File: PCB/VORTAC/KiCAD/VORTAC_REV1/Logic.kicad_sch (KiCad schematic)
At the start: 28 parts, among them U1 TLV73333PDBV, U3 EE-SX3350, U4 TPS54335ADRCR, U7 EE-SX3350

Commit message: Fixed Library stuff
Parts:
- L2: footprint ToolChanger:L_Sunlord_MWSA0518_5.4x5.2mm -> Vortac:L_Sunlord_MWSA0518_5.4x5.2mm; LCSC C408412 -> C436530; LCSC ALT C436530 -> (none)
- U3, U7: footprint ToolChanger:SENSOR_EE-SX3350_OMR -> Vortac:SENSOR_EE-SX3350_OMR
- U4: footprint ToolChanger:VSON-10-1EP_3x3mm_P0.5mm_EP1.65x2.4mm_ThermalVias -> Vortac:VSON-10-1EP_3x3mm_P0.5mm_EP1.65x2.4mm_ThermalVias
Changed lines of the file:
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@@
 			)
 		)
-		(property "Footprint" "ToolChanger:L_Sunlord_MWSA0518_5.4x5.2mm"
+		(property "Footprint" "Vortac:L_Sunlord_MWSA0518_5.4x5.2mm"
 			(at 82.55 116.84 0)
 			(effects
@@
 			)
 		)
-		(property "LCSC" "C408412"
-			(at 82.55 116.84 90)
-			(effects
-				(font
-					(size 1.27 1.27)
-				)
-				(hide yes)
-			)
-		)
-		(property "LCSC ALT" "C436530"
+		(property "LCSC" "C436530"
 			(at 82.55 116.84 90)
 			(effects
@@
 			)
 		)
-		(property "Footprint" "ToolChanger:VSON-10-1EP_3x3mm_P0.5mm_EP1.65x2.4mm_ThermalVias"
+		(property "Footprint" "Vortac:VSON-10-1EP_3x3mm_P0.5mm_EP1.65x2.4mm_ThermalVias"
 			(at 66.04 133.35 0)
 			(effects
@@
 			)
 		)
-		(property "Footprint" "ToolChanger:SENSOR_EE-SX3350_OMR"
+		(property "Footprint" "Vortac:SENSOR_EE-SX3350_OMR"
 			(at 214.884 67.564 0)
 			(effects
@@
 			)
 		)
-		(property "Footprint" "ToolChanger:SENSOR_EE-SX3350_OMR"
+		(property "Footprint" "Vortac:SENSOR_EE-SX3350_OMR"
 			(at 214.884 44.704 0)
 			(effects

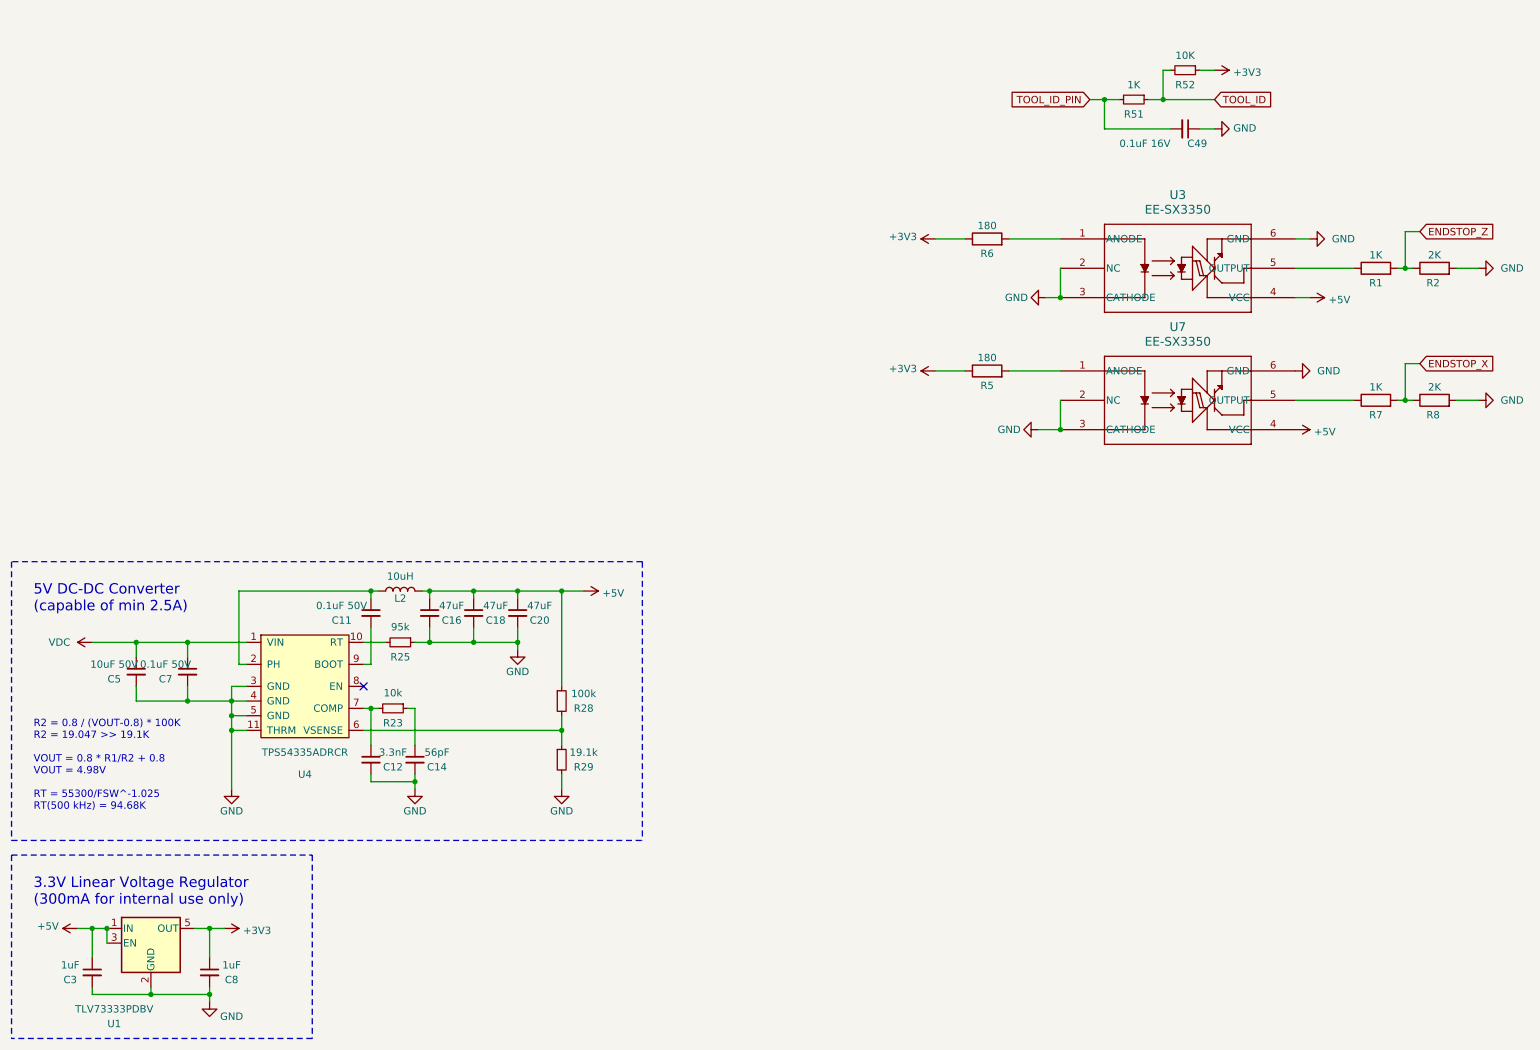
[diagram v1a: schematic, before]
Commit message: pls merge Jenno
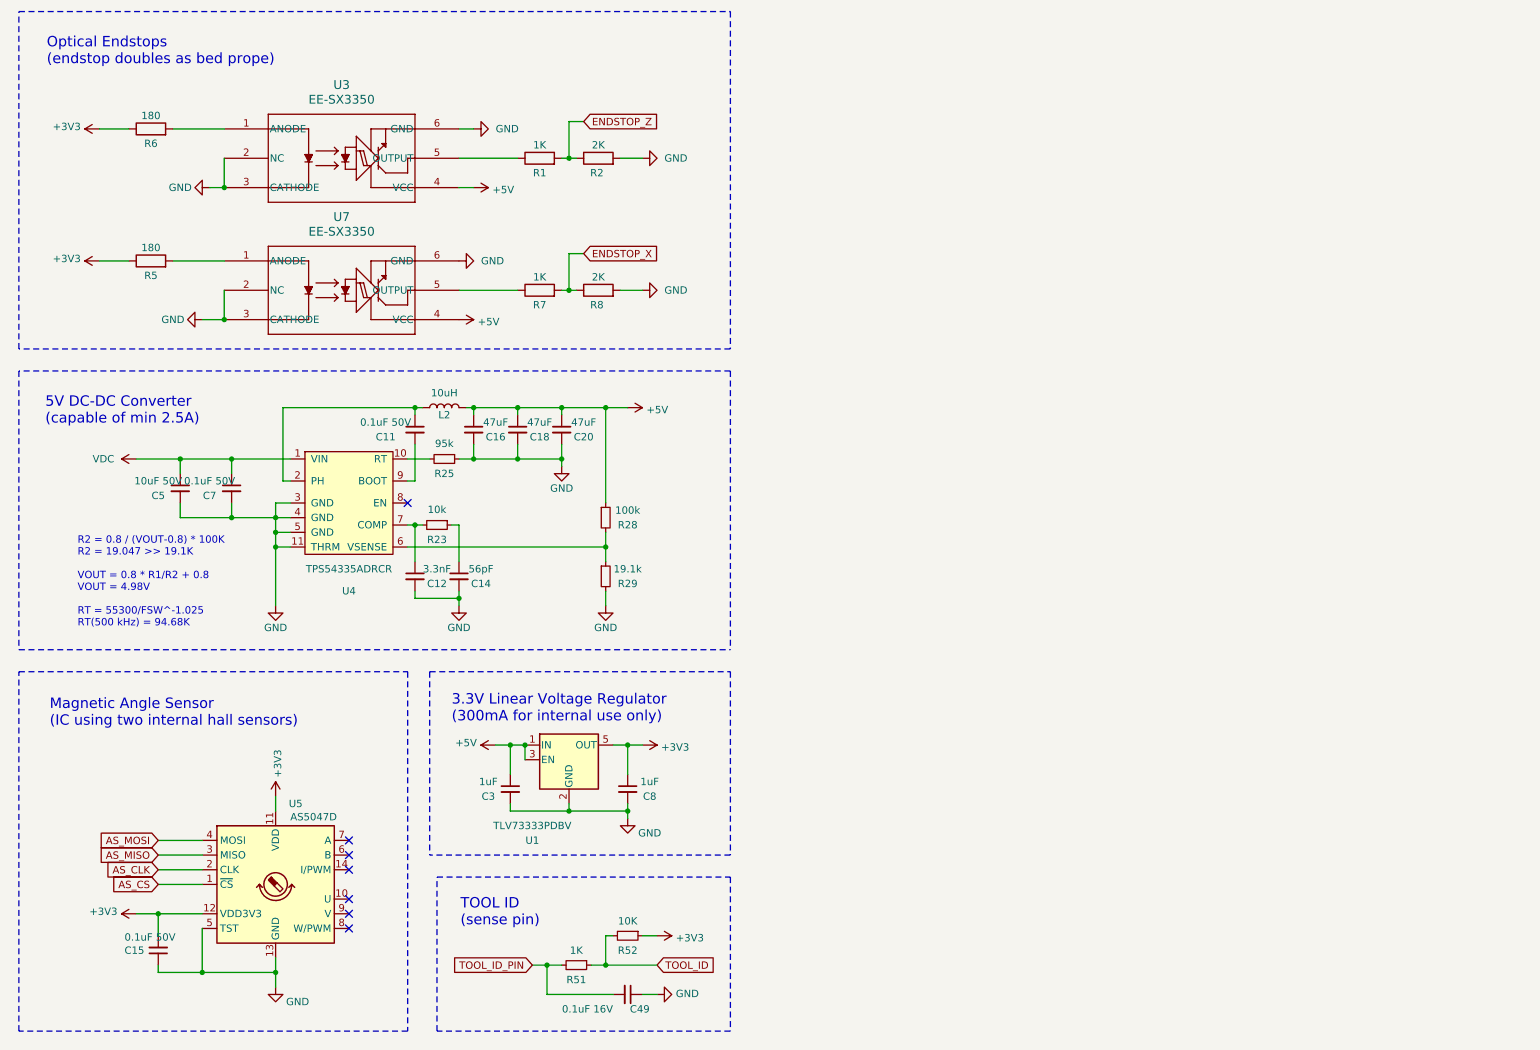
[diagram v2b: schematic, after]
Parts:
- added C15: 0.1uF 50V, Capacitor_SMD:C_0603_1608Metric, symbol Device:C_Small
- added U5: AS5047D, Package_SO:TSSOP-14_4.4x5mm_P0.65mm, symbol Sensor_Magnetic:AS5047D
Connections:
- net +3V3: now also C15.2, U5.11 (VDD), U5.12 (VDD3V3)
- net GND: now also C15.1, U5.13 (GND), U5.5 (TST)
- new net AS_CLK: U5.2 (CLK)
- new net AS_CS: U5.1 (~{CS})
- new net AS_MISO: U5.3 (MISO)
- new net AS_MOSI: U5.4 (MOSI)
- no-connect marks 1 -> 7
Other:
- note added: "Magnetic Angle Sensor (IC using two internal hall sensors)"
- note added: "Optical Endstops (endstop doubles as bed prope)"
- note added: "TOOL ID (sense pin)"
- moved on the sheet: C11, C12, C14, C16, C18, C20, C3, C49, C5, C7, C8, L2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
